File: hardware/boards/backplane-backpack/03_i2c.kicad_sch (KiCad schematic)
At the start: 13 parts, among them J11 backplane_mate, U2 TCA9548APWR

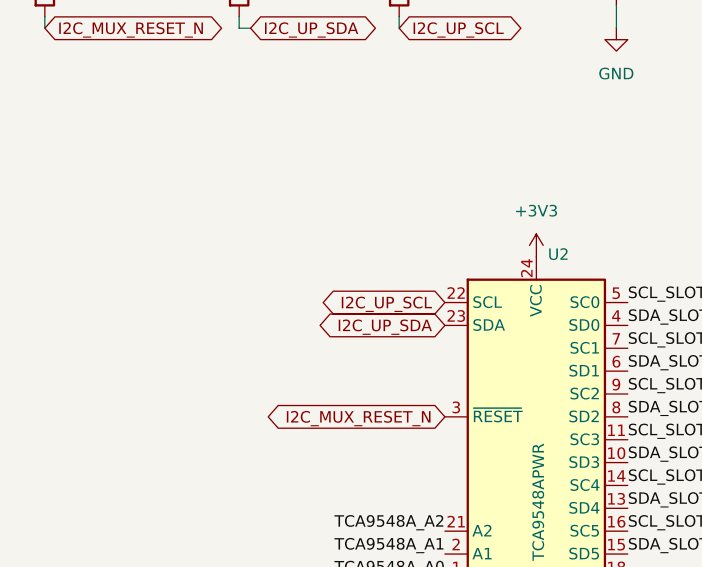
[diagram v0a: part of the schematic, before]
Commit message: chore: checkpoint current board layout
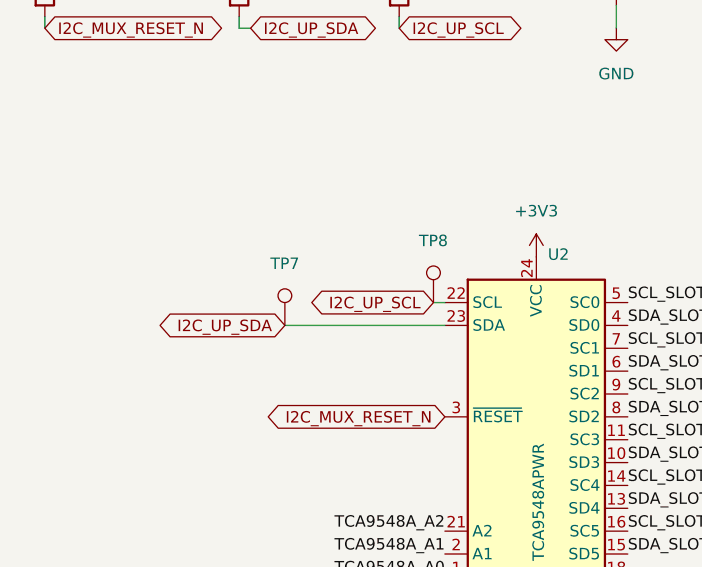
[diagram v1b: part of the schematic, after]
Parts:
- added TP7: I2C_UP_SDA, TestPoint:TestPoint_Pad_D1.5mm, symbol Connector:TestPoint
- added TP8: I2C_UP_SCL, TestPoint:TestPoint_Pad_D1.5mm, symbol Connector:TestPoint
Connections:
- net I2C_UP_SCL: now also TP8.1
- net I2C_UP_SDA: now also TP7.1
